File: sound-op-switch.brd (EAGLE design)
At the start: 50 x 50 mm, 35 parts, among them IC1 PIC12F1822, IC2 LM358D

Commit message: add device names and bom
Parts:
- C1: value (none) -> 4u7
- C3: value (none) -> 100u
- R1, R2, R3, R4, R5: value (none) -> 10k
- R10, R11, R9: value (none) -> 2k2
- R12: value 10k -> 1k
- R13: value (none) -> 1m
- R6: value (none) -> 470
- R7, R8: value 10k -> 2k2
- T1: value (none) -> MMBTA13
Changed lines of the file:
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@@
 <attribute name="VALUE" x="9.017" y="23.114" size="1.27" layer="27" rot="R90"/>
 </element>
-<element name="R7" library="resistor" package="R0805" value="10k" x="13.97" y="26.67" smashed="yes">
+<element name="R7" library="resistor" package="R0805" value="2k2" x="13.97" y="26.67" smashed="yes">
 <attribute name="NAME" x="15.24" y="29.083" size="1.27" layer="25" rot="R180"/>
 </element>
-<element name="R12" library="rcl" package="R0805" value="10k" x="20.32" y="3.81" smashed="yes" rot="R180">
+<element name="R12" library="rcl" package="R0805" value="1k" x="20.32" y="3.81" smashed="yes" rot="R180">
 <attribute name="NAME" x="22.0726" y="2.4638" size="1.27" layer="25" rot="R180"/>
 </element>
@@
 <attribute name="NAME" x="12.3444" y="15.9512" size="1.27" layer="21" rot="R90"/>
 </element>
-<element name="R13" library="resistor" package="R0805" value="" x="38.1" y="3.81" smashed="yes" rot="R180">
+<element name="R13" library="resistor" package="R0805" value="1m" x="38.1" y="3.81" smashed="yes" rot="R180">
 <attribute name="NAME" x="39.8272" y="2.4892" size="1.27" layer="25" rot="R180"/>
 <attribute name="VALUE" x="38.862" y="6.096" size="1.27" layer="27" rot="R180"/>
@@
 <attribute name="VALUE" x="35.179" y="48.641" size="1.27" layer="27" rot="R180"/>
 </element>
-<element name="R6" library="resistor" package="R0805" value="" x="36.449" y="30.734" smashed="yes" rot="R180">
+<element name="R6" library="resistor" package="R0805" value="470" x="36.449" y="30.734" smashed="yes" rot="R180">
 <attribute name="NAME" x="40.894" y="31.369" size="1.27" layer="25" rot="R180"/>
 <attribute name="VALUE" x="37.211" y="33.02" size="1.27" layer="27" rot="R180"/>
@@
 <attribute name="VALUE" x="36.449" y="23.495" size="1.27" layer="27" ratio="10" rot="R270"/>
 </element>
-<element name="R11" library="resistor" package="R0805" value="" x="41.91" y="25.4" smashed="yes" rot="R270">
+<element name="R11" library="resistor" package="R0805" value="2k2" x="41.91" y="25.4" smashed="yes" rot="R270">
 <attribute name="NAME" x="40.3098" y="28.6512" size="1.27" layer="25"/>
 <attribute name="VALUE" x="39.624" y="26.162" size="1.27" layer="27" rot="R270"/>
@@
 <attribute name="NAME" x="14.9606" y="40.894" size="1.27" layer="21" rot="R270"/>
 </element>
-<element name="R5" library="resistor" package="R0805" value="" x="31.369" y="30.734" smashed="yes">
+<element name="R5" library="resistor" package="R0805" value="10k" x="31.369" y="30.734" smashed="yes">
 <attribute name="NAME" x="28.321" y="28.321" size="1.27" layer="25"/>
 <attribute name="VALUE" x="30.607" y="28.448" size="1.27" layer="27"/>
@@
 <attribute name="NAME" x="22.7076" y="30.353" size="1.27" layer="21" rot="R180"/>
 </element>
-<element name="R1" library="resistor" package="R0805" value="" x="20.32" y="46.609" smashed="yes">
+<element name="R1" library="resistor" package="R0805" value="10k" x="20.32" y="46.609" smashed="yes">
 <attribute name="NAME" x="19.558" y="47.625" size="1.27" layer="25"/>
 <attribute name="VALUE" x="19.558" y="44.323" size="1.27" layer="27"/>
 </element>
-<element name="R4" library="resistor" package="R0805" value="" x="25.4" y="35.56" smashed="yes">
+<element name="R4" library="resistor" package="R0805" value="10k" x="25.4" y="35.56" smashed="yes">
 <attribute name="NAME" x="24.1808" y="33.0708" size="1.27" layer="25"/>
 <attribute name="VALUE" x="24.638" y="33.274" size="1.27" layer="27"/>
 </element>
-<element name="R3" library="resistor" package="R0805" value="" x="25.4" y="39.37" smashed="yes" rot="R180">
+<element name="R3" library="resistor" package="R0805" value="10k" x="25.4" y="39.37" smashed="yes" rot="R180">
 <attribute name="NAME" x="25.6032" y="38.1254" size="1.27" layer="25" rot="R180"/>
 <attribute name="VALUE" x="26.162" y="41.656" size="1.27" layer="27" rot="R180"/>
@@
 <attribute name="NAME" x="32.385" y="32.639" size="1.27" layer="25" ratio="10"/>
 </element>
-<element name="R8" library="resistor" package="R0805" value="10k" x="13.97" y="23.876" smashed="yes">
+<element name="R8" library="resistor" package="R0805" value="2k2" x="13.97" y="23.876" smashed="yes">
 <attribute name="NAME" x="12.954" y="21.463" size="1.27" layer="25"/>
 </element>
-<element name="C3" library="rcl" package="E2,5-6E" value="" x="12.7" y="3.81" smashed="yes" rot="R270">
+<element name="C3" library="rcl" package="E2,5-6E" value="100u" x="12.7" y="3.81" smashed="yes" rot="R270">
 <attribute name="NAME" x="8.128" y="0.635" size="1.27" layer="25" ratio="10"/>
 <attribute name="VALUE" x="10.16" y="1.143" size="1.27" layer="27" ratio="10" rot="R270"/>
@@
 <attribute name="VALUE" x="18.669" y="23.495" size="1.27" layer="27" ratio="10" rot="R270"/>
 </element>
-<element name="R9" library="resistor" package="R0805" value="" x="24.13" y="25.4" smashed="yes" rot="R270">
+<element name="R9" library="resistor" package="R0805" value="2k2" x="24.13" y="25.4" smashed="yes" rot="R270">
 <attribute name="NAME" x="24.3078" y="21.5138" size="1.27" layer="25"/>
 <attribute name="VALUE" x="21.844" y="26.162" size="1.27" layer="27" rot="R270"/>
@@
 <attribute name="VALUE" x="27.559" y="23.495" size="1.27" layer="27" ratio="10" rot="R270"/>
 </element>
-<element name="R10" library="resistor" package="R0805" value="" x="33.02" y="25.4" smashed="yes" rot="R270">
+<element name="R10" library="resistor" package="R0805" value="2k2" x="33.02" y="25.4" smashed="yes" rot="R270">
 <attribute name="NAME" x="31.877" y="28.702" size="1.27" layer="25"/>
 <attribute name="VALUE" x="30.734" y="26.162" size="1.27" layer="27" rot="R270"/>
 </element>
-<element name="R2" library="resistor" package="R0805" value="" x="25.4" y="41.91" smashed="yes">
+<element name="R2" library="resistor" package="R0805" value="10k" x="25.4" y="41.91" smashed="yes">
 <attribute name="NAME" x="24.4348" y="43.1038" size="1.27" layer="25"/>
 <attribute name="VALUE" x="24.638" y="39.624" size="1.27" layer="27"/>
 </element>
-<element name="C1" library="rcl" package="E2,5-6E" value="" x="26.035" y="46.355" smashed="yes" rot="R180">
+<element name="C1" library="rcl" package="E2,5-6E" value="4u7" x="26.035" y="46.355" smashed="yes" rot="R180">
 <attribute name="NAME" x="29.083" y="47.371" size="1.27" layer="25" ratio="10" rot="R270"/>
 <attribute name="VALUE" x="23.368" y="48.895" size="1.27" layer="27" ratio="10" rot="R180"/>
@@
 <attribute name="VALUE" x="50.927" y="22.86" size="1.27" layer="27" rot="R90"/>
 </element>
-<element name="T1" library="transistor-neu-to92" package="SOT23-BEC" value="" x="25.4" y="29.845" smashed="yes" rot="R90">
+<element name="T1" library="transistor-neu-to92" package="SOT23-BEC" value="MMBTA13" x="25.4" y="29.845" smashed="yes" rot="R90">
 <attribute name="NAME" x="26.1112" y="32.7406" size="1.27" layer="25" rot="R180"/>
 <attribute name="VALUE" x="28.575" y="27.94" size="1.27" layer="27" rot="R90"/>

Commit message: case proto
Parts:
- C3: value 100u -> 1u
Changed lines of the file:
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@@
 <attribute name="NAME" x="12.954" y="21.463" size="1.27" layer="25"/>
 </element>
-<element name="C3" library="rcl" package="E2,5-6E" value="100u" x="12.7" y="3.81" smashed="yes" rot="R270">
+<element name="C3" library="rcl" package="E2,5-6E" value="1u" x="12.7" y="3.81" smashed="yes" rot="R270">
 <attribute name="NAME" x="8.128" y="0.635" size="1.27" layer="25" ratio="10"/>
 <attribute name="VALUE" x="10.16" y="1.143" size="1.27" layer="27" ratio="10" rot="R270"/>

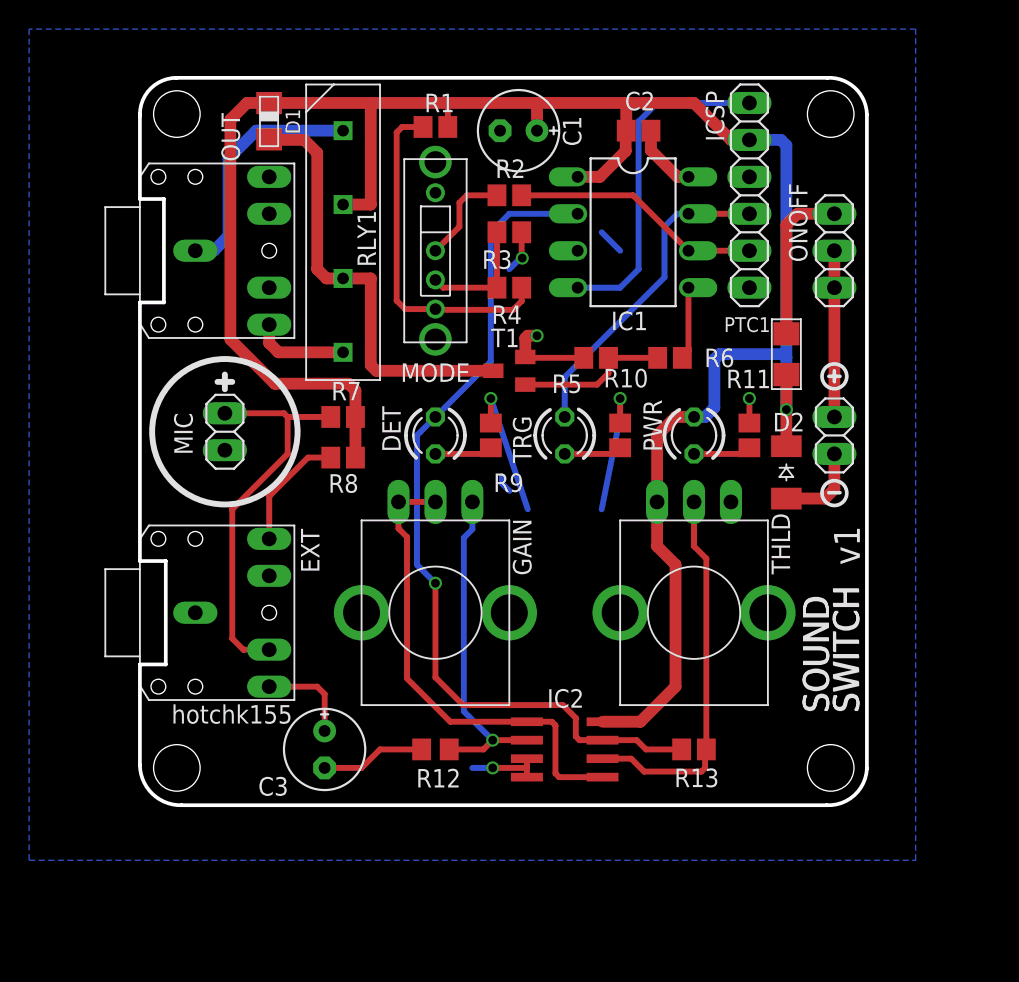
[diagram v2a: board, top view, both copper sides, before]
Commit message: pcb rev2
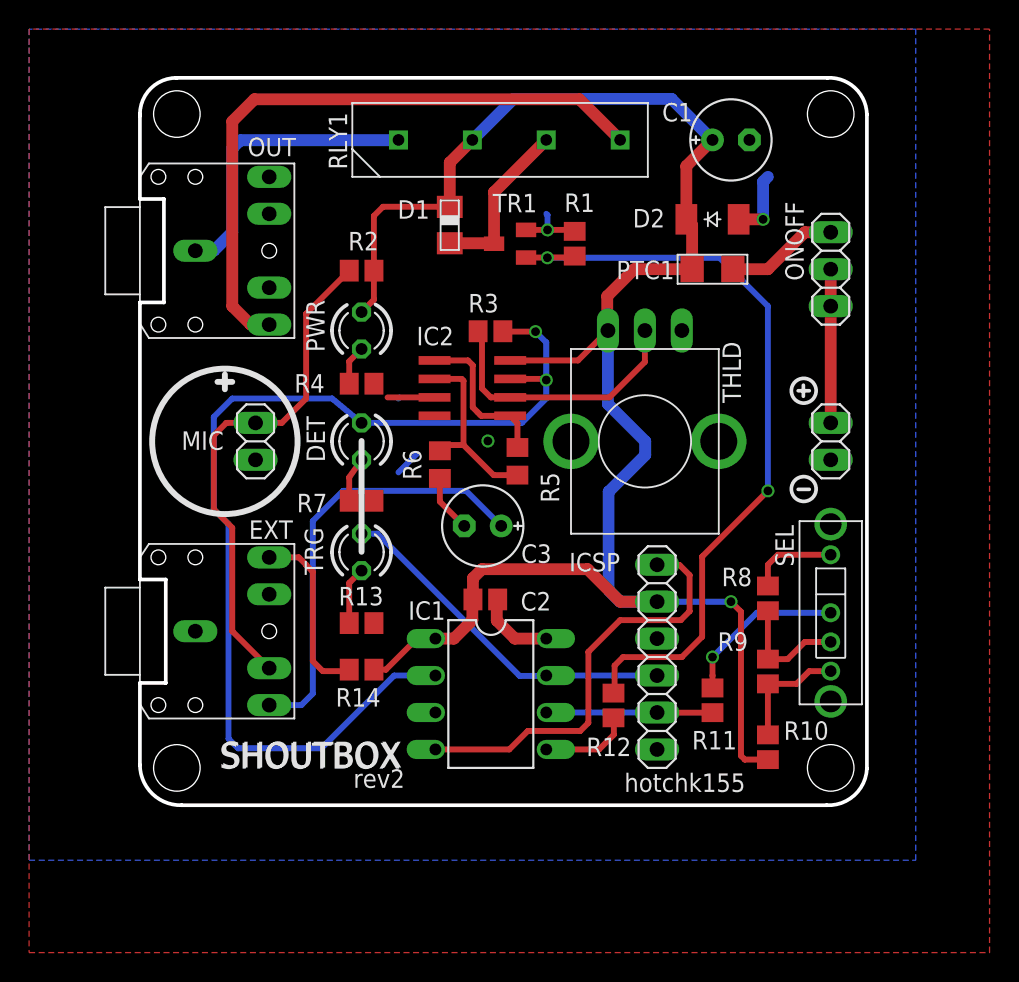
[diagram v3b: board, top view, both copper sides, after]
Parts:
- removed GAIN: ALPS_POT_SMALL, jasons_stuff:SMALL_ALPS_POT
- removed MODE: SP4T-SLIDE, jason_eagle6:SP3T-SLIDE
- removed T1: MMBTA13, transistor-neu-to92:SOT23-BEC
- added R14: 2k2, resistor:R0805
- added SEL: SP4T-SLIDE, jason_eagle6:SP3T-SLIDE
- added TR1: MMBTA13, transistor-neu-to92:SOT23-BEC
- R10, R11, R8, R9: value 2k2 -> 10k
- R12: value 1k -> 470; device rcl:R0805 -> resistor:R0805
- R13: value 1m -> 2k2
- R2, R4: value 10k -> 2k2
- R3: value 10k -> 1m
- R5: value 10k -> 100k; device resistor:R0805 -> rcl:R0805
- R6: value 470 -> 1k; device resistor:R0805 -> rcl:R0805
- moved C2 33.9 mm to (23.7, 14.1)
- moved IC1 33.2 mm to (24.1, 7.62)
- moved ICSP 32.4 mm to (35.6, 10.2)
- moved R8 30.8 mm to (43.2, 14.2), turned to 270 degrees
- moved IC2 25.6 mm to (22.9, 28.7)
- moved R9 25.0 mm to (43.2, 9.17)
- moved R13 24.5 mm to (15.2, 12.5)
- moved PWR 24.0 mm to (15.2, 32.6)
- moved R10 23.7 mm to (43.2, 3.96)
- moved C3 18.8 mm to (23.6, 19.2), turned to 180 degrees
- moved R11 18.4 mm to (39.4, 7.19)
- moved D2 18.1 mm to (39.4, 40.3), turned to 0 degrees
- moved R6 17.4 mm to (20.6, 23.4), turned to 270 degrees
- moved TRG 16.1 mm to (15.2, 17.4)
- moved C1 14.6 mm to (40.6, 45.7), turned to 0 degrees
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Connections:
- net GND: now also R1.1, R13.1, R4.1, R7.1, R8.1, SEL.1, TR1.E; no longer MODE.1, R10.1, R11.1, R3.1, R5.1, R9.1, T1.E
- net INPUT: now also R3.2; no longer R13.2
- net N$1: now also R2.1; no longer R7.1
- net N$10: now also R1.2, R12.2, TR1.B; no longer R5.2, R6.2, T1.B
- net N$13: now also R3.1; no longer R13.1
- net N$14: now also R8.2, R9.1, SEL.3; no longer MODE.3, R3.2, R4.1
- net N$15: now also TR1.C; no longer T1.C
- net N$16: now also R4.2; no longer R11.2
- net N$17: now also R13.2; no longer R10.2
- net N$2: now also R6.2; no longer R12.2
- net N$3: now also R5.2, R6.1; no longer GAIN.A, R12.1
- net N$4: now also R7.2; no longer R9.2
- net N$5: now also R14.1; no longer R8.1
- net N$7: now also R5.1; no longer GAIN.B, GAIN.W
- net N$8: now also R10.1, R9.2, SEL.4; no longer MODE.4, R1.1, R4.2
- net N$9: now also R11.2; no longer R2.2
- net OUTPUT: now also R12.1; no longer R6.1
- net VCC: now also R10.2, R14.2, R2.2; no longer R1.2, R7.2, R8.2
- net VSEL: now also R11.1, SEL.2; no longer MODE.2, R2.1
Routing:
- net N$10: track 10.5 -> 53.3 mm, vias 0 -> 2
- net N$28: track 6.61 -> 44.2 mm
- net N$12: track 6.56 -> 30.0 mm
- net GND: track 49.4 -> 26.2 mm, vias 6 -> 3
- net N$7: track 33.1 -> 10.9 mm
- net VCC: track 149.8 -> 129.4 mm
- net N$15: track 30.2 -> 11.7 mm
- net N$8: track 23.6 -> 8.19 mm
- net INPUT: track 59.5 -> 72.2 mm, vias 1 -> 2
- net N$3: track 23.0 -> 12.8 mm, vias 1 -> 0
- net N$1: track 27.1 -> 35.0 mm
- net N$13: track 26.2 -> 18.7 mm
- net N$11: track 23.0 -> 29.3 mm
- net N$9: track 17.2 -> 11.4 mm
- net VSEL: track 6.78 -> 11.5 mm, vias 0 -> 1
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- added copper zone on layer 1, net GND
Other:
- outline, holes or cut-outs redrawn
- board text added: "SHOUTBOX"
- board text added: "rev2"
- board text removed: "SOUND"
- board text removed: "SWITCH"
- board text removed: "v1"
